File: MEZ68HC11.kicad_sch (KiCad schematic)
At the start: 22 parts, among them J1 Conn_01x20_Socket, J2 Conn_01x20_Socket, J3 Conn_01x08_Socket, J4 Conn_01x06_Socket, J5 Conn_01x08_Socket, U1 68HC11_PLCC, U2 74HC573, Y1 8MHz

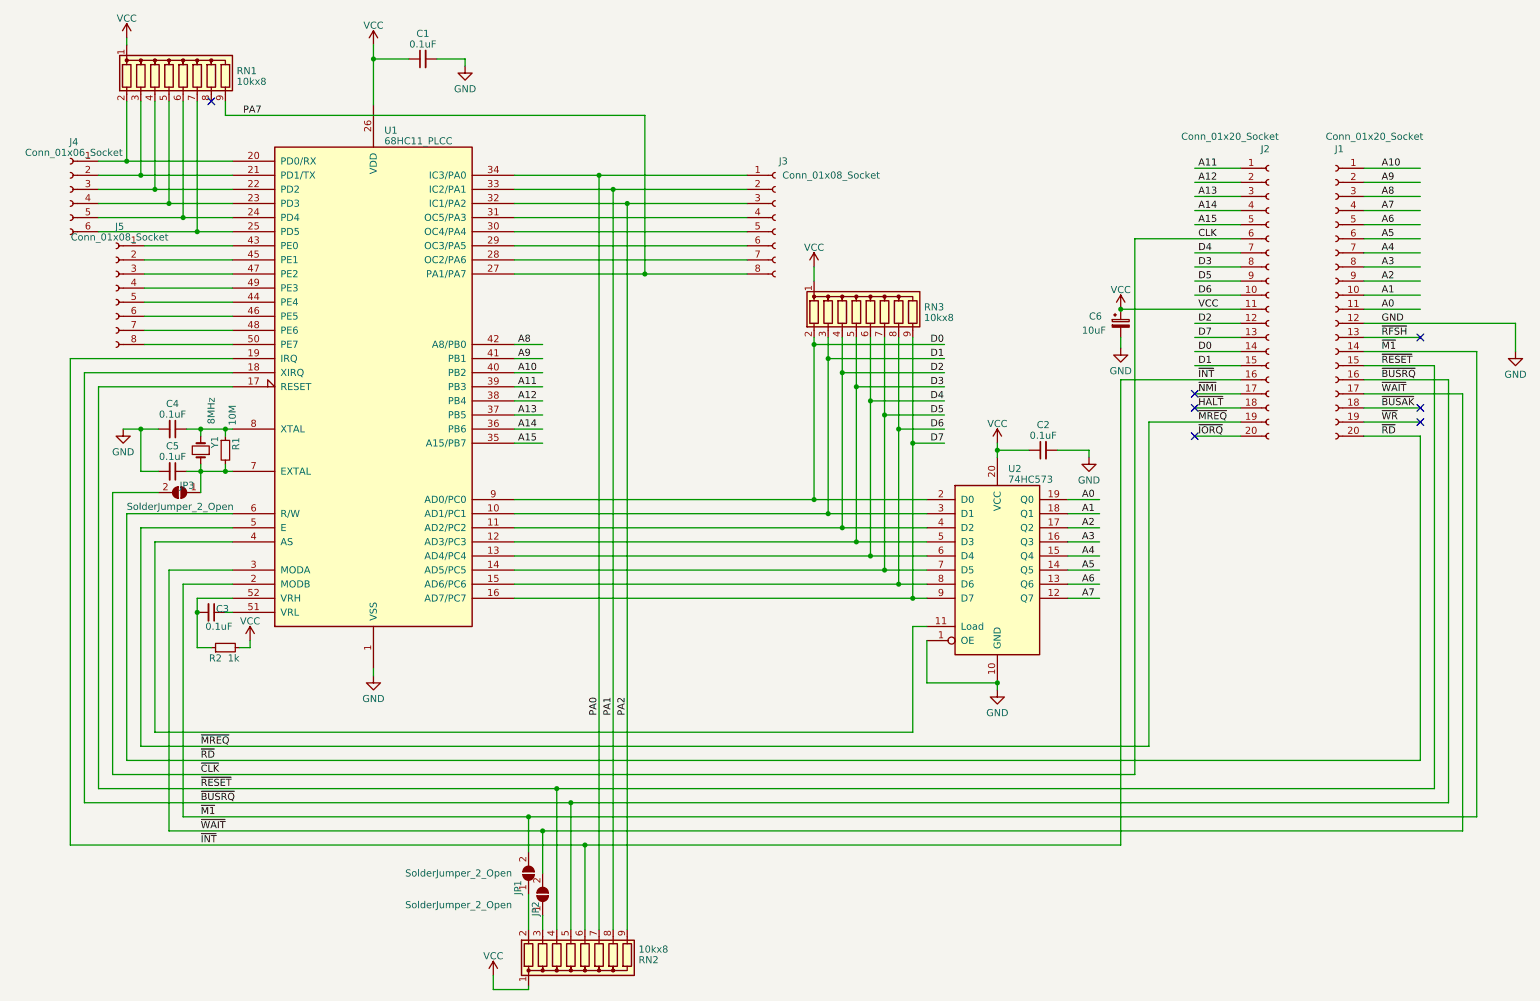
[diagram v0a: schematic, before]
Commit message: add some in the schematics
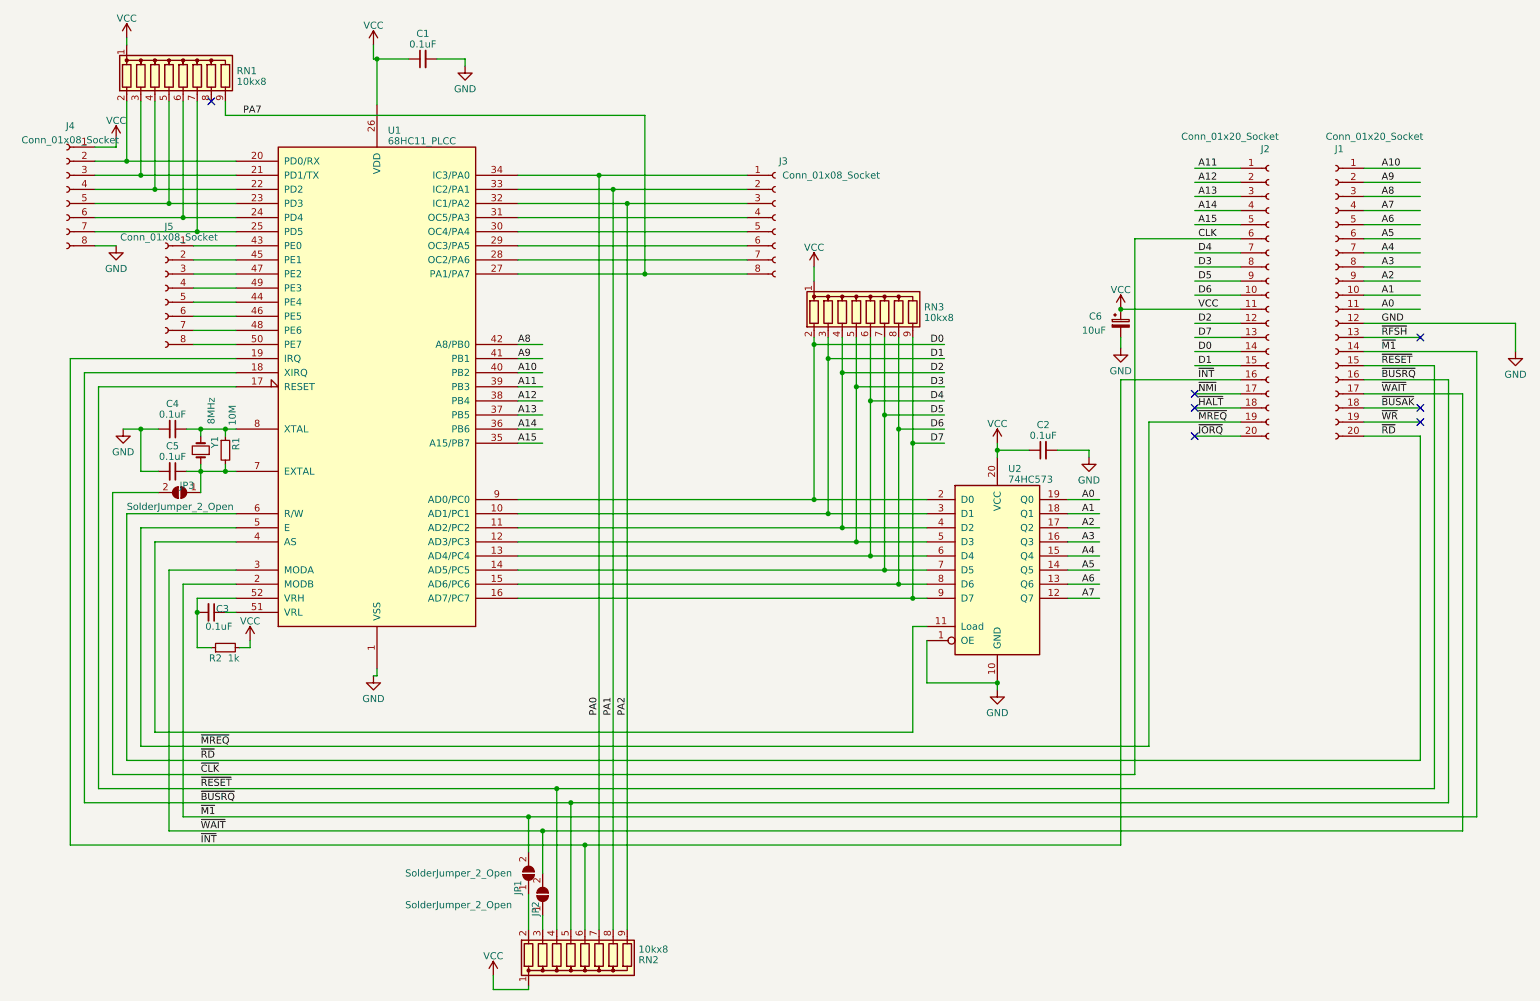
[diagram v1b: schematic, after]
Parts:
- removed J4: Conn_01x06_Socket, symbol Connector:Conn_01x06_Socket
- added J4: Conn_01x08_Socket, symbol Connector:Conn_01x08_Socket
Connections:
- net GND: now also J4.8 (Pin_8)
- net VCC: now also J4.1 (Pin_1)
- net at RN1.2 (R1), U1.20 (PD0/RX): now also J4.2 (Pin_2)
- net at RN1.3 (R2), U1.21 (PD1/TX): now also J4.3 (Pin_3)
- net at RN1.4 (R3), U1.22 (PD2): now also J4.4 (Pin_4)
- net at RN1.5 (R4), U1.23 (PD3): now also J4.5 (Pin_5)
- net at RN1.6 (R5), U1.24 (PD4): now also J4.6 (Pin_6)
- net at RN1.7 (R6), U1.25 (PD5): now also J4.7 (Pin_7)
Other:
- moved on the sheet: J5, U1
